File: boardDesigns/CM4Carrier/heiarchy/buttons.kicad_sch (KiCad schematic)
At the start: 84 parts, among them J2 Conn_01x04_Female, J7 Conn_01x03_Male, SW1 SW_Push, SW10 SW_Push, SW11 SW_Push, SW13 SW_Push, SW14 SW_Push, SW15 SW_Push, SW2 SW_Push, SW3 SW_Push, SW4 SW_Push, SW5 SW_Push, SW6 SW_Push, SW7 SW_Push, SW8 SW_Push, SW9 SW_Push, U5 74HC00, U6 MCP3002

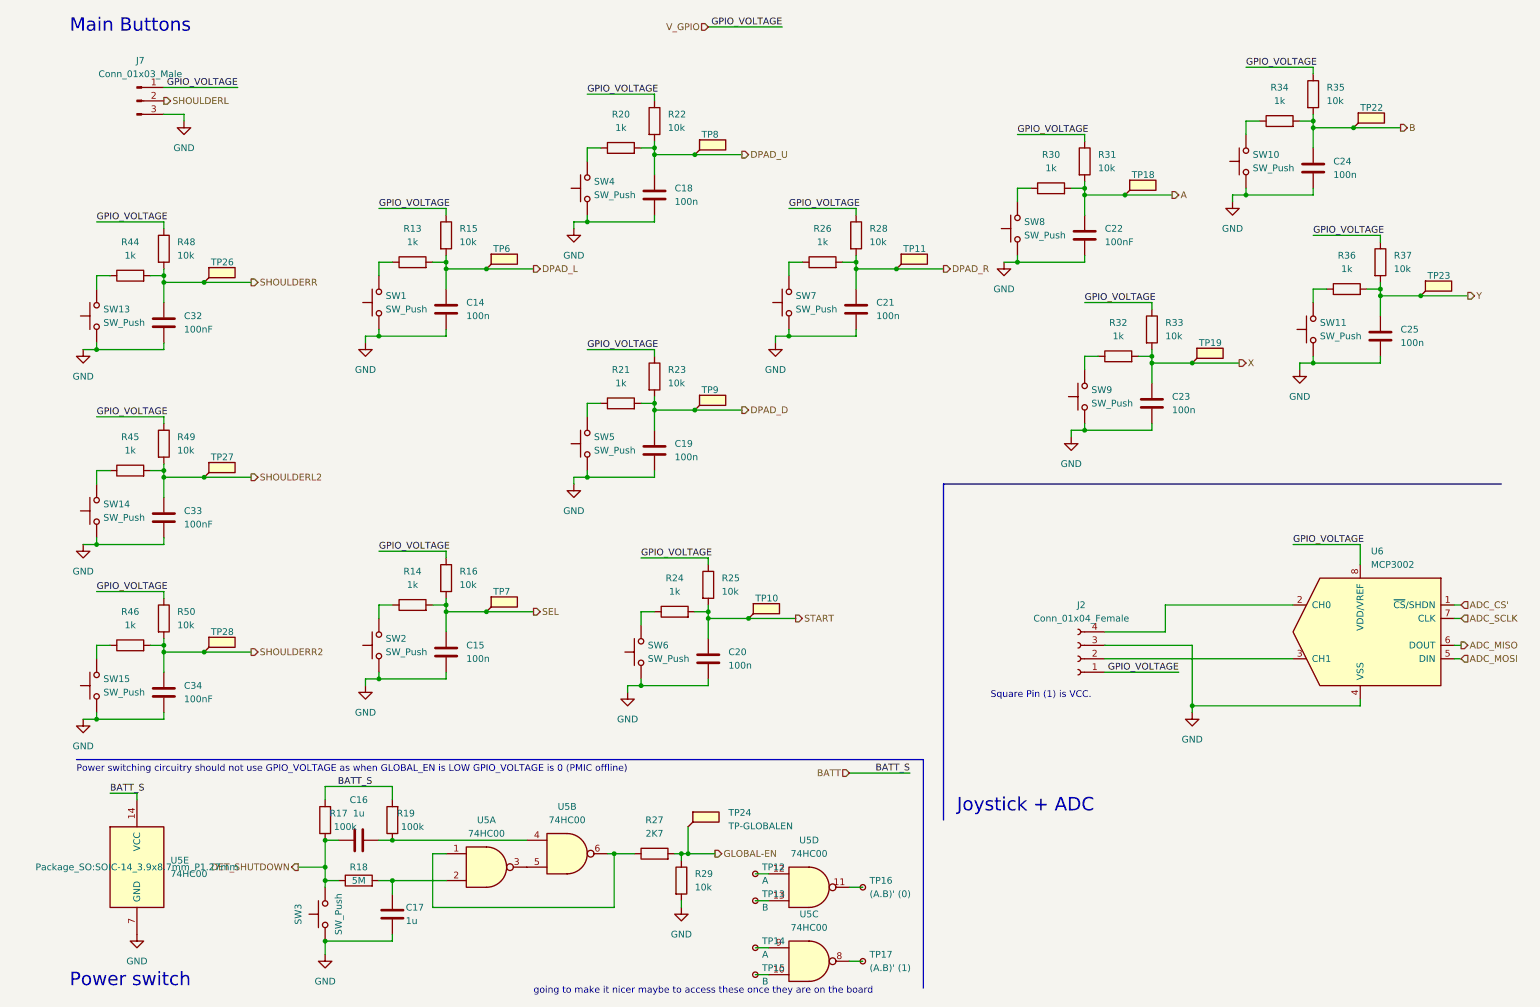
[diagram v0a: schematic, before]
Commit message: rev1
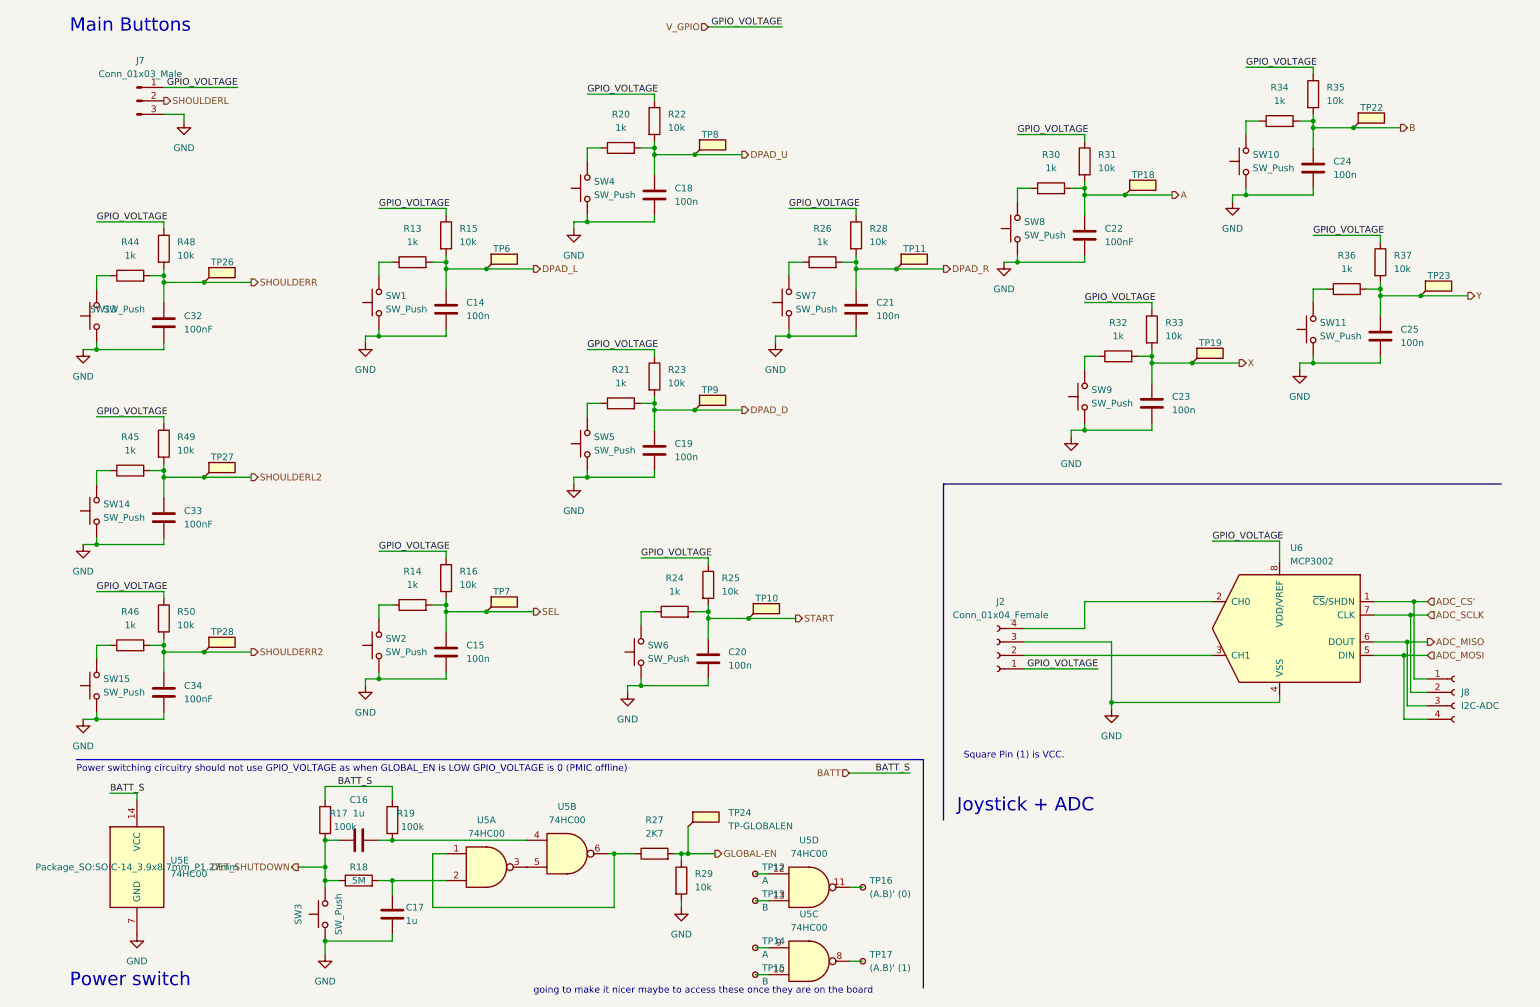
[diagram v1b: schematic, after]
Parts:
- added J8: I2C-ADC, Connector_Wire:SolderWire-0.1sqmm_1x04_P3.6mm_D0.4mm_OD1mm, symbol Connector:Conn_01x04_Female
- SW13: footprint CM4IO:SW_PTS526_SMG15_SMTR2_LFS -> CM4IO:SW_EVQ-P7J01P
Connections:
- net ADC_CS': now also J8.1 (Pin_1)
- net ADC_MISO: now also J8.3 (Pin_3)
- net ADC_MOSI: now also J8.4 (Pin_4)
- net ADC_SCLK: now also J8.2 (Pin_2)
- net GND: now also SW13.1_1 (1), SW13.1_2 (1); no longer SW13.1
- net at R44.1: now also SW13.2_1 (2), SW13.2_2 (2); no longer SW13.2
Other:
- moved on the sheet: J2, U6
